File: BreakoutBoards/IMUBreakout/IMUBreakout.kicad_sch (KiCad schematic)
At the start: 14 parts, among them J10 IMU Connection, J5 Qwicc, U1 ICM-20948, U2 MIC5504-1.8YM5

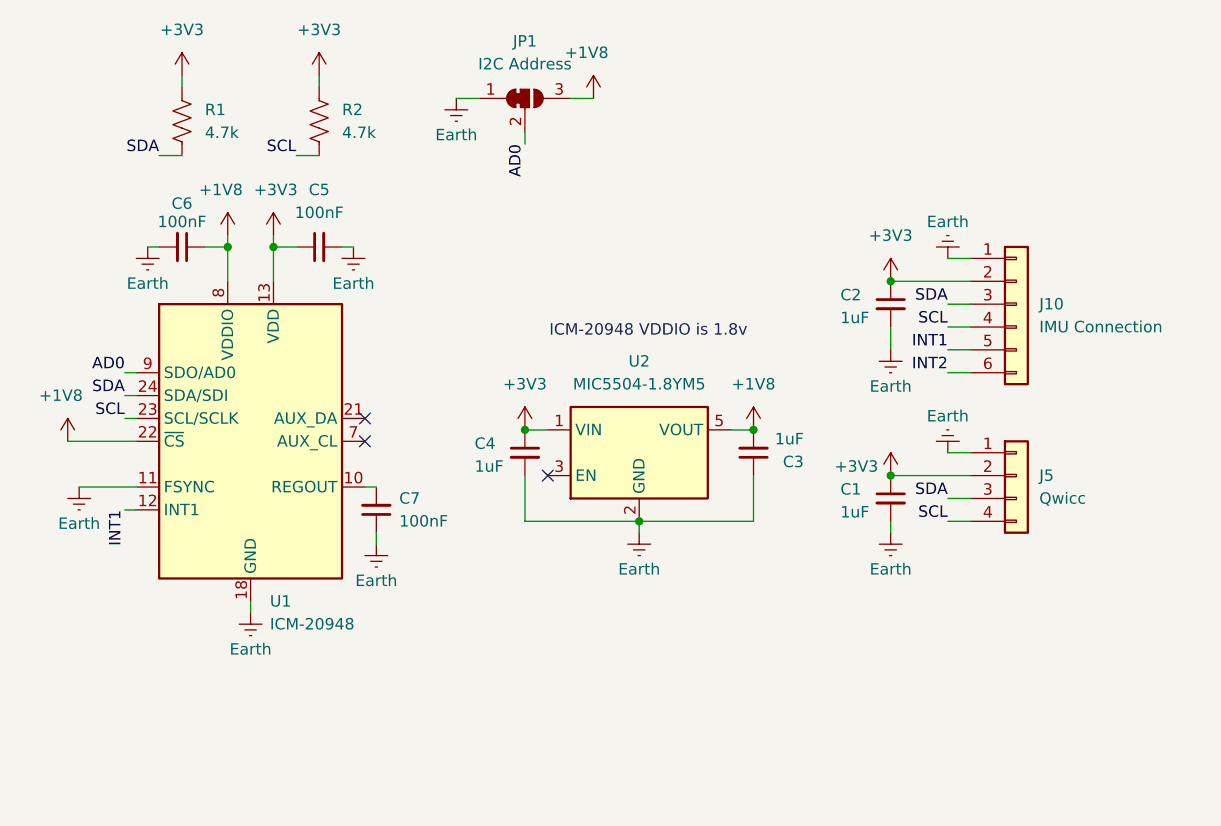
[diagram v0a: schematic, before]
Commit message: updated IMU board and production files
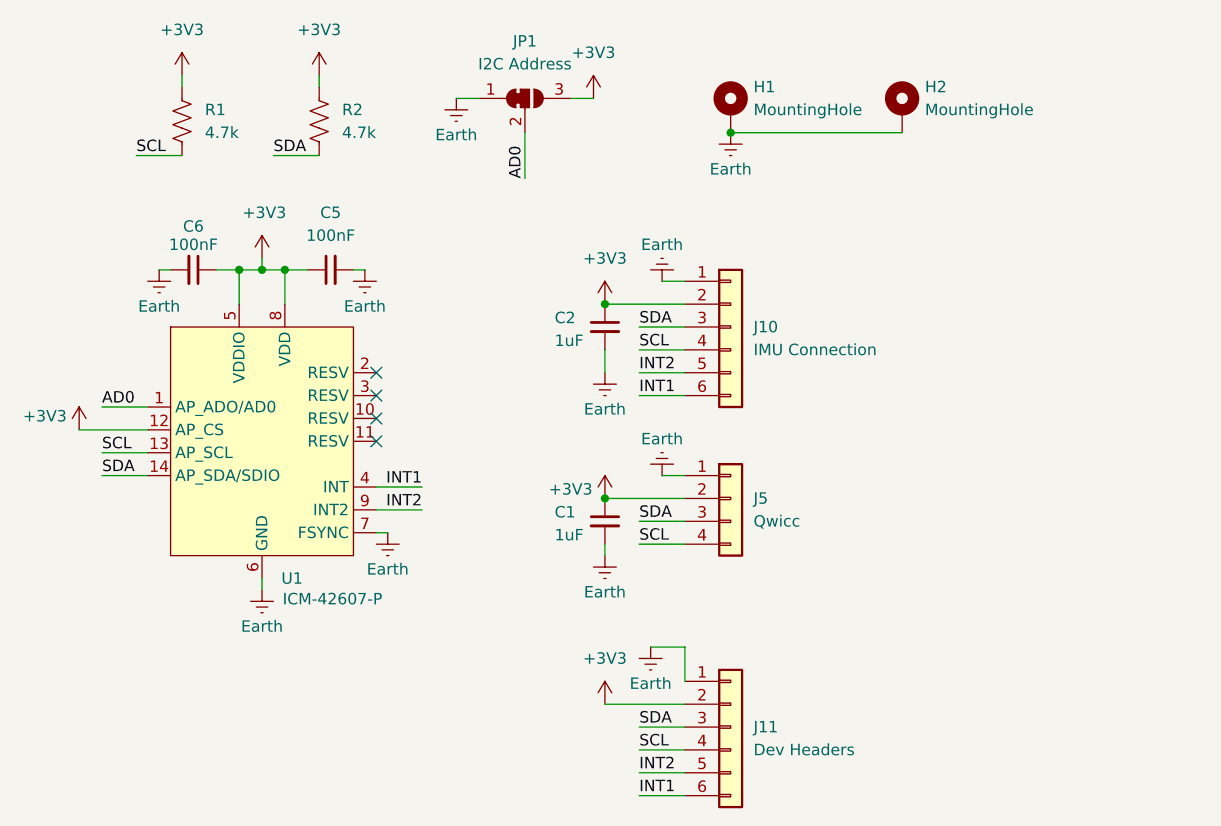
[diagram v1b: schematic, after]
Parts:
- removed C3, C4: 1uF, Capacitor_SMD:C_0603_1608Metric, symbol Device:C_Small
- removed C7: 100nF, Capacitor_SMD:C_0603_1608Metric, symbol Device:C_Small
- removed U1: ICM-20948, Sensor_Motion:InvenSense_QFN-24_3x3mm_P0.4mm, symbol Sensor_Motion:ICM-20948
- removed U2: MIC5504-1.8YM5, Package_TO_SOT_SMD:SOT-23-5, symbol Regulator_Linear:MIC5504-1.8YM5
- added H1, H2: MountingHole, MountingHole:MountingHole_2.2mm_M2_Pad_Via, symbol Mechanical:MountingHole_Pad
- added J11: Dev Headers, Connector_PinSocket_2.54mm:PinSocket_1x06_P2.54mm_Vertical, symbol Connector_Generic:Conn_01x06
- added U1: ICM-42607-P, Package_LGA:Bosch_LGA-14_3x2.5mm_P0.5mm, symbol IMUBreakout:ICM-42607-P
- C1, C2: footprint Capacitor_SMD:C_0603_1608Metric -> Capacitor_SMD:C_0402_1005Metric; LCSC (none) -> C52923
- C5, C6: footprint Capacitor_SMD:C_0603_1608Metric -> Capacitor_SMD:C_0402_1005Metric; LCSC (none) -> C1525
- J10: LCSC (none) -> C160405
- J5: LCSC (none) -> C51940130
- R1, R2: footprint Resistor_SMD:R_0603_1608Metric -> Resistor_SMD:R_0402_1005Metric; LCSC (none) -> C25900
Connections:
- net +1V8 is gone; now on net +3V3: C6.1, JP1.3 (B)
- net +3V3: now also J11.2 (Pin_2), U1.12 (AP_CS), U1.5 (VDDIO), U1.8 (VDD)
- net AD0: now also U1.1 (AP_ADO/AD0)
- net Earth: now also H1.1, H2.1, J11.1 (Pin_1), U1.6 (GND), U1.7 (FSYNC)
- net INT1: now also J10.6 (Pin_6), J11.6 (Pin_6), U1.4 (INT); no longer J10.5 (Pin_5)
- net INT2: now also J10.5 (Pin_5), J11.5 (Pin_5), U1.9 (INT2); no longer J10.6 (Pin_6)
- net SCL: now also R1.2, J11.4 (Pin_4), U1.13 (AP_SCL); no longer R2.2
- net SDA: now also R2.2, J11.3 (Pin_3), U1.14 (AP_SDA/SDIO); no longer R1.2
- no-connect marks 3 -> 4
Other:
- note removed: "ICM-20948 VDDIO is 1.8v"
- moved on the sheet: C1, C2, C5, C6, J10, J5
